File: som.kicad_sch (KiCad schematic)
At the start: 33 parts, among them J1 Bus_DDR4_SODIMM_CUSTOM_Jetson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, U1 NTS0102

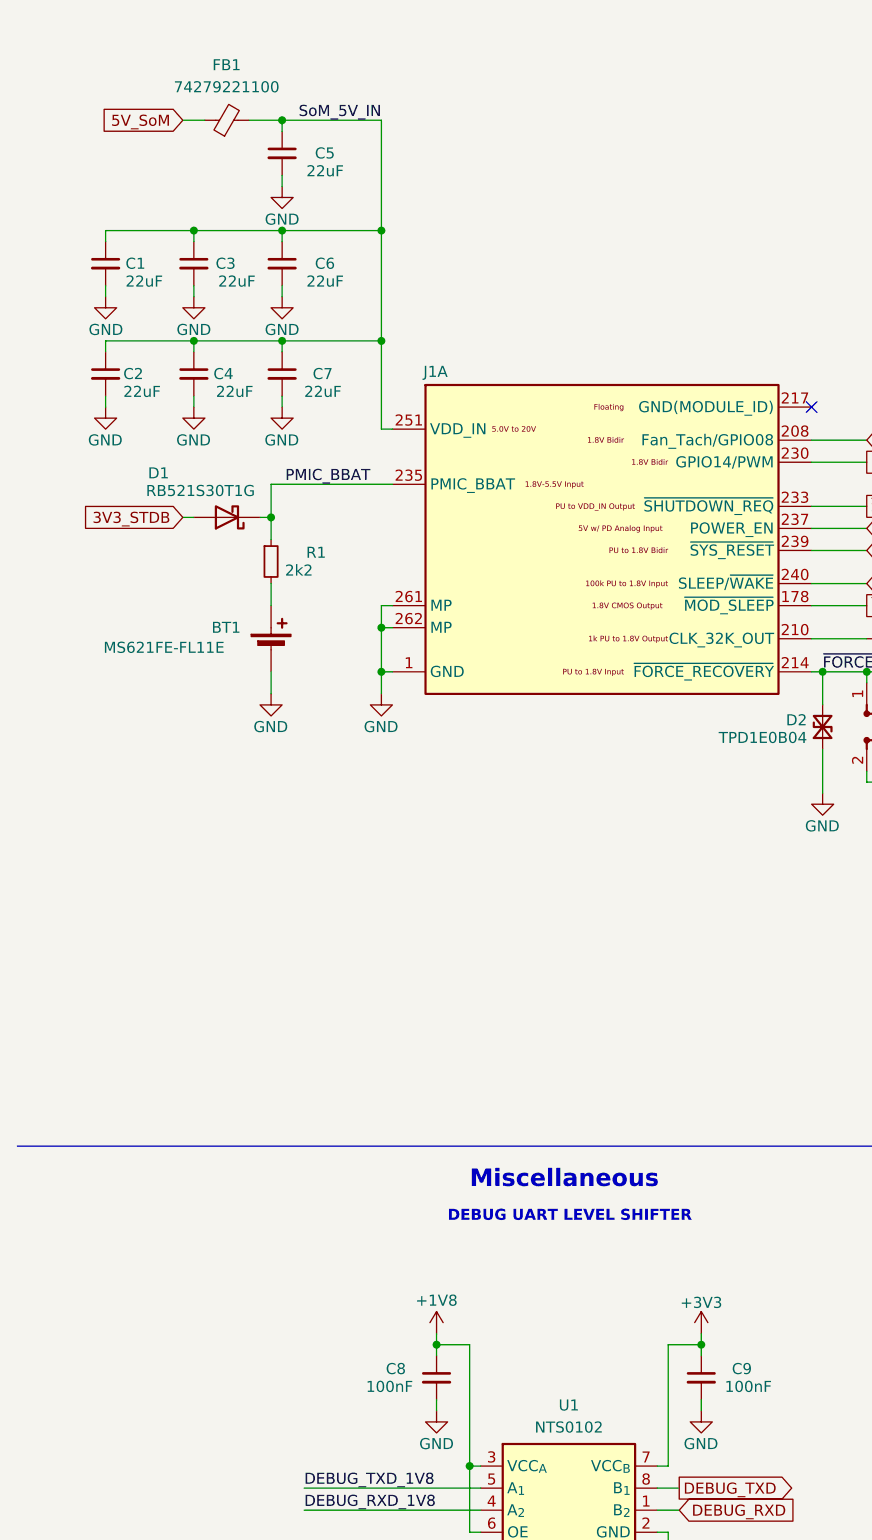
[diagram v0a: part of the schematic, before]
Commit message: Final BOM changes, gerbers
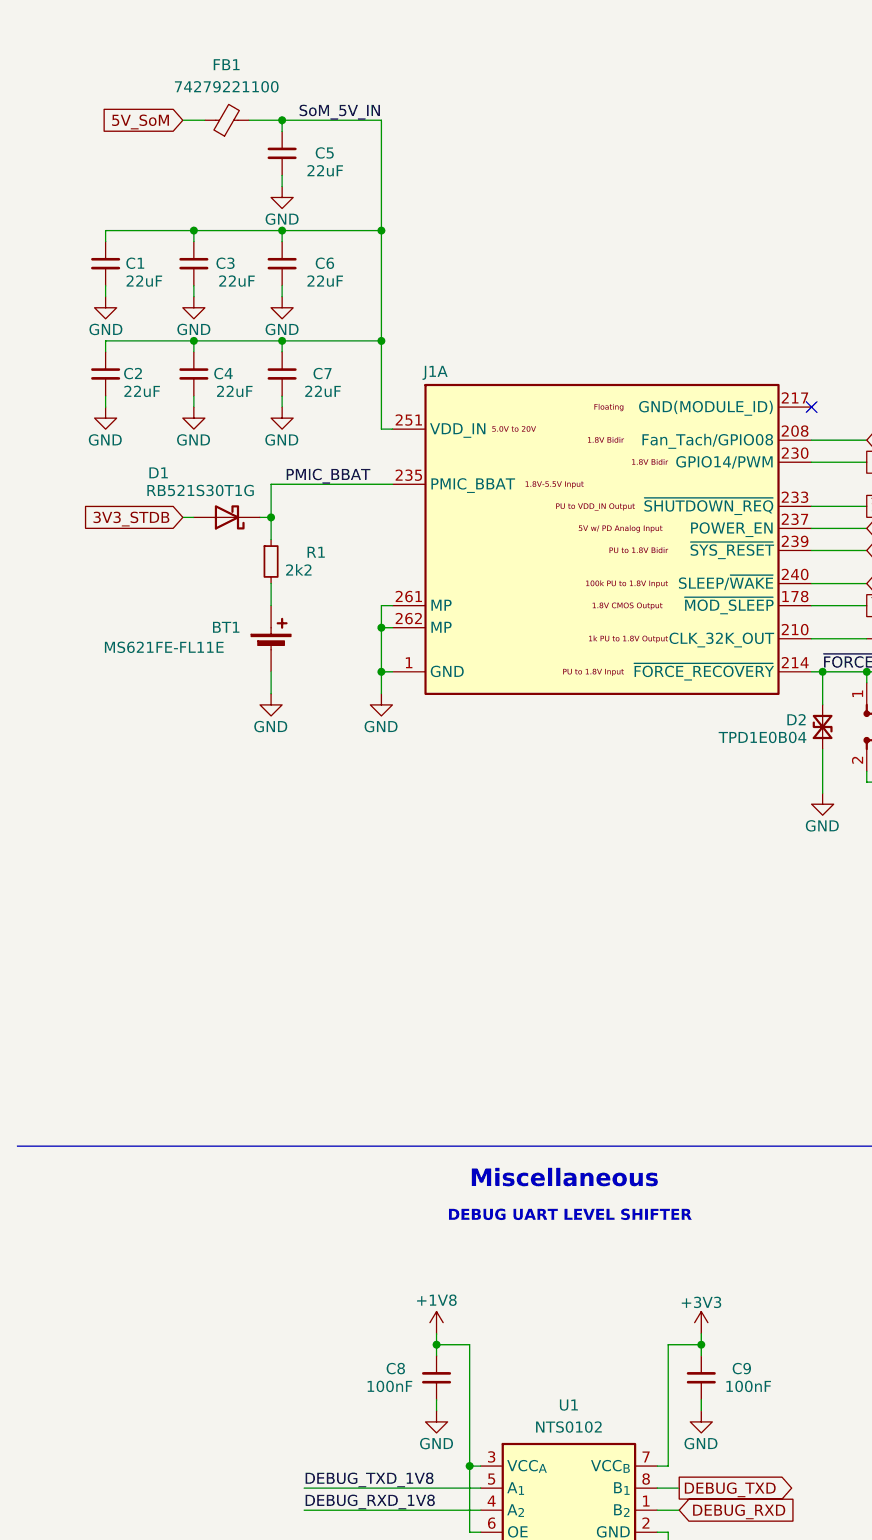
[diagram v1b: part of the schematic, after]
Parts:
- BTN1: LCSC (none) -> C221676
- C1, C2, C3, C4, C5, C6, C7: LCSC (none) -> C84419
- C8, C9: LCSC (none) -> C14663
- D1: LCSC (none) -> C145179
- D2: LCSC (none) -> C1975594
- FB1: LCSC (none) -> C5355985
- J1: LCSC (none) -> C5164025
- R1: LCSC (none) -> C4190
- R10, R11, R12, R13, R14, R15, R2, R3, R4, R5, R6, R7, R8, R9: LCSC (none) -> C17168
- U1: LCSC (none) -> C2687851
